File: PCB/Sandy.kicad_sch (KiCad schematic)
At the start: 156 parts, among them J1 USB_C_Receptacle_USB2.0, J2 Conn_01x03, J3 Conn_01x02, J4 Conn_02x03_Odd_Even, J5 Conn_02x02_Top_Bottom, J6 Conn_02x02_Top_Bottom, J7 Conn_02x02_Top_Bottom, J8 Conn_02x02_Top_Bottom, U1 ATmega32U4-MU, U2 24LC64, Y1 16MHz

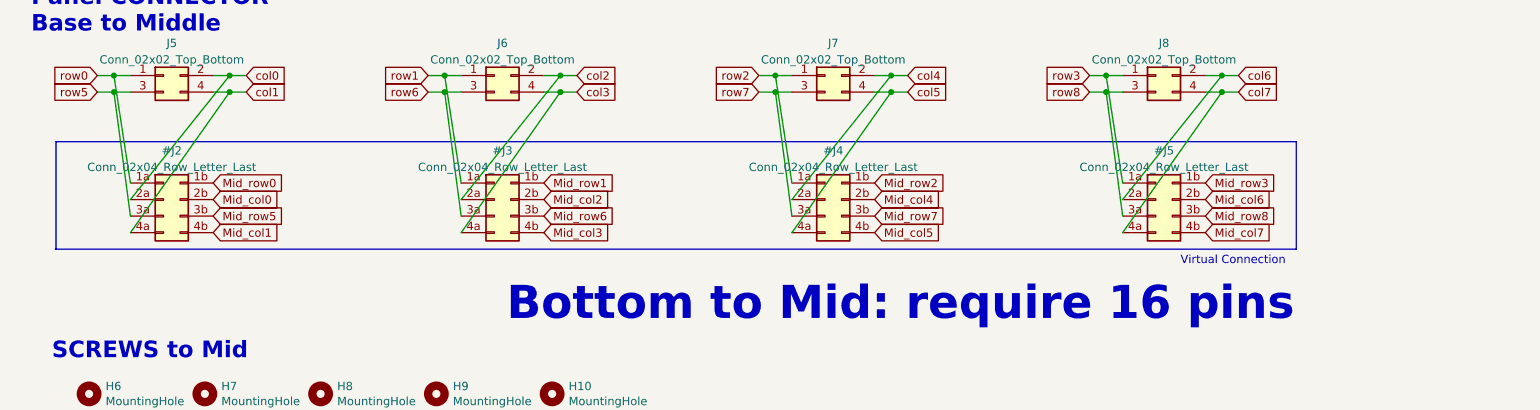
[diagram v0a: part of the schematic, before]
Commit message: コネクタ位置考え中
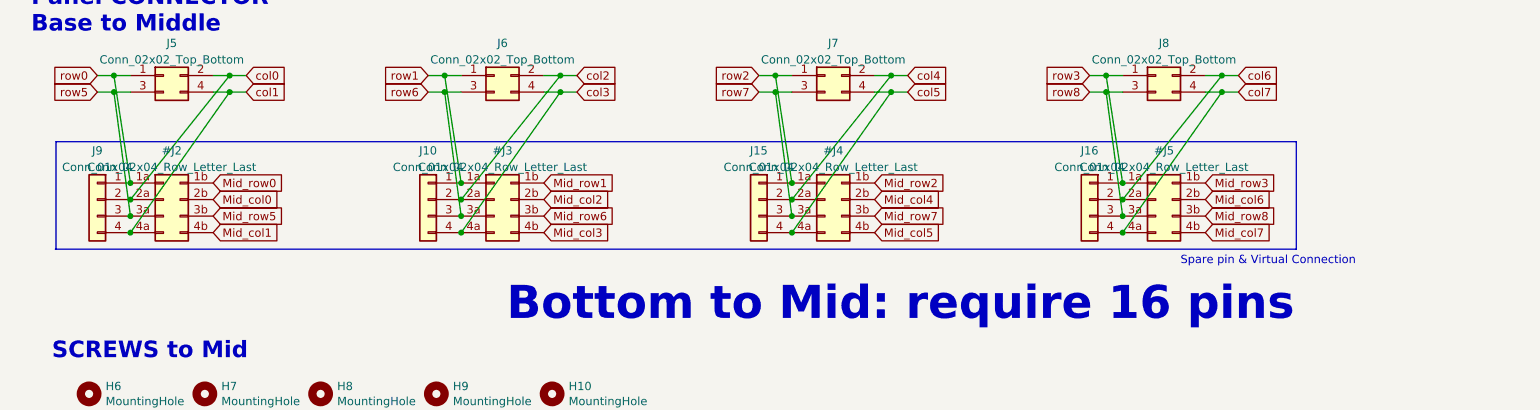
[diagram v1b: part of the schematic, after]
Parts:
- added J10, J15, J16, J9: Conn_01x04, Connector_PinHeader_2.54mm:PinHeader_1x04_P2.54mm_Vertical, symbol Connector_Generic:Conn_01x04
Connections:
- net MISO: now also J10.4 (Pin_4)
- net MOSI: now also J10.2 (Pin_2)
- net RE_L1_1: now also J9.2 (Pin_2)
- net RE_R1_1: now also J16.4 (Pin_4)
- net RE_R2_1: now also J15.2 (Pin_2)
- net SCK: now also J9.4 (Pin_4)
- net col5: now also J15.4 (Pin_4)
- net col6: now also J16.2 (Pin_2)
- net row0: now also J9.1 (Pin_1)
- net row1: now also J10.1 (Pin_1)
- net row2: now also J15.1 (Pin_1)
- net row3: now also J16.1 (Pin_1)
- net row5: now also J9.3 (Pin_3)
- net row6: now also J10.3 (Pin_3)
- net row7: now also J15.3 (Pin_3)
- net row8: now also J16.3 (Pin_3)
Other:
- note added: "Spare pin & Virtual Connection"
- note removed: "Virtual Connection"
